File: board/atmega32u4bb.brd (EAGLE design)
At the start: 30.4 x 12.2 mm, 18 parts, among them X3 16MHz

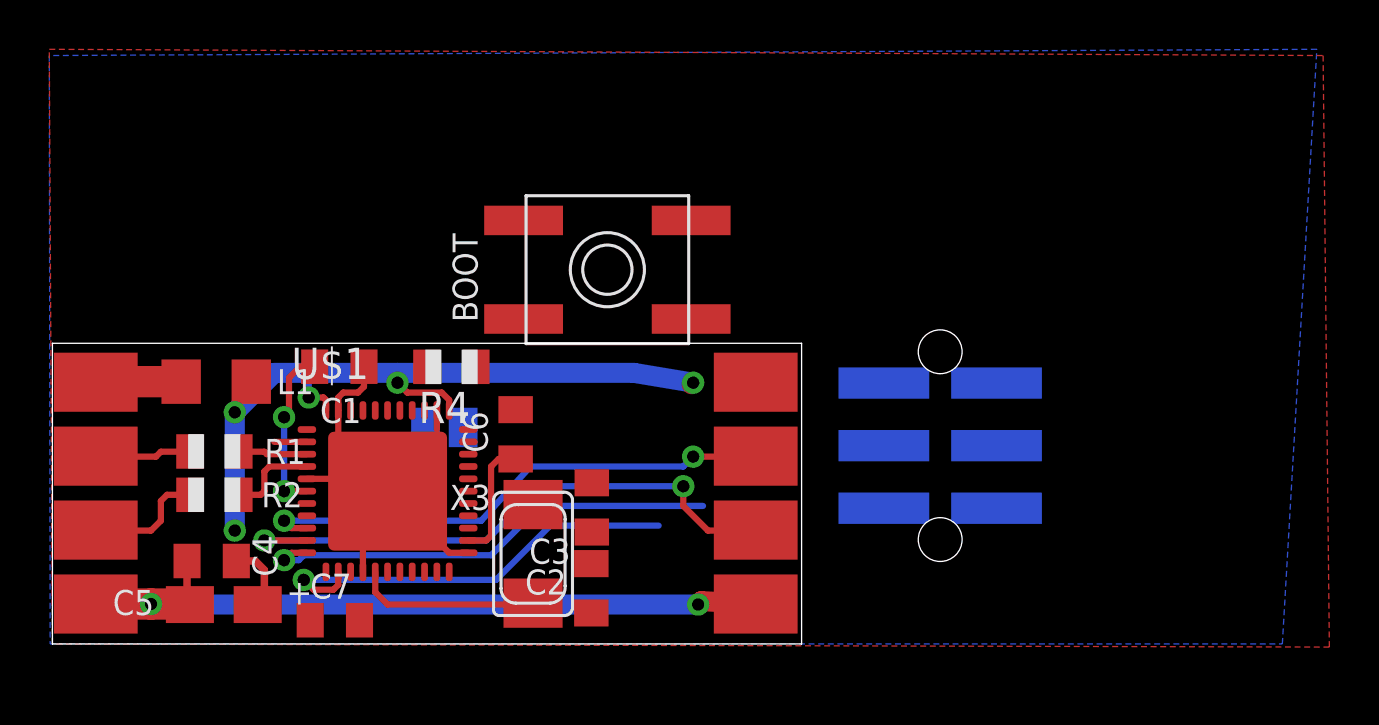
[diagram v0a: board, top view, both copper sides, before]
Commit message: V1 board design
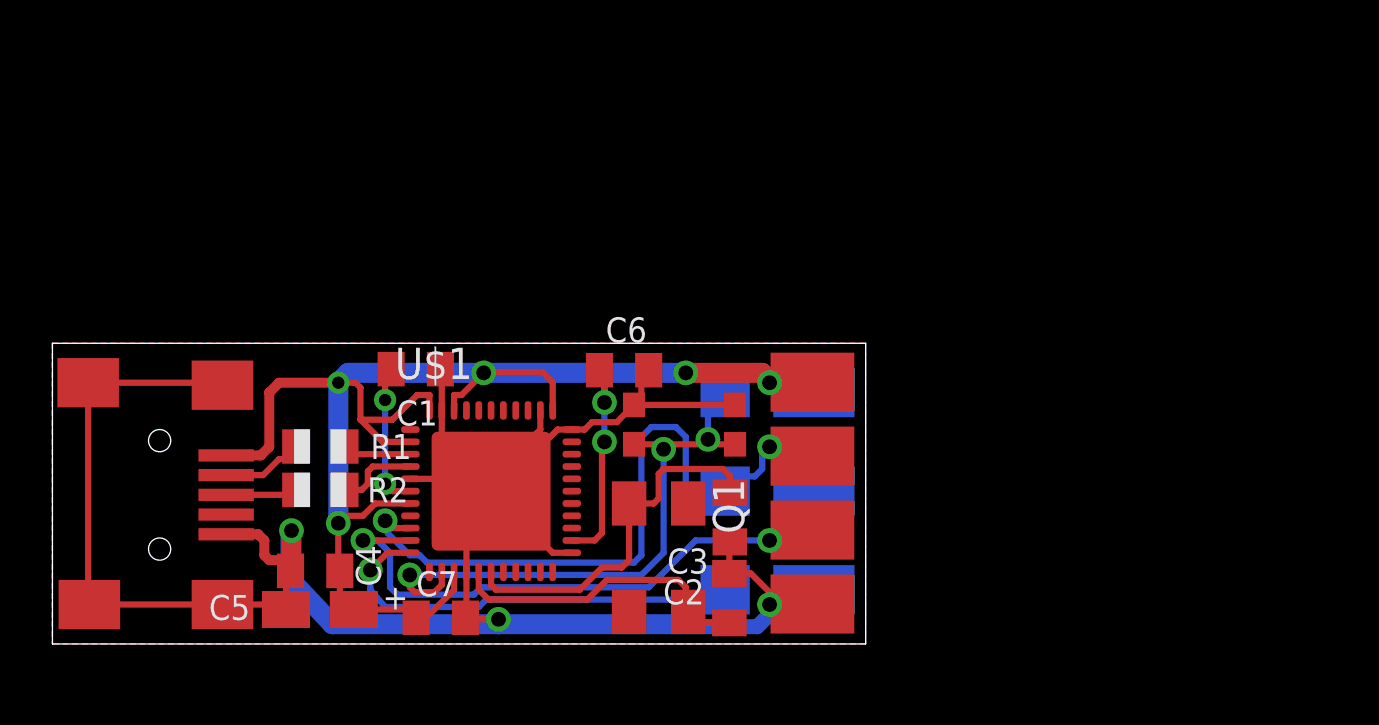
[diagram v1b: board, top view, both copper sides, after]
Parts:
- removed BOOT: EVQQ2, adaprog:EVQ-Q2
- removed ISP6: PINHD-2X3, adaprog:2X3SMT
- removed L1: 500mA, adafruit:R1206
- removed R4: 10K, adafruit:R0805
- removed SJ1: HWB, jumper:SJ
- removed U$5: USB_PADS, glowboard:PAD_CONNECTION
- removed X3: 16MHz, adaprog:NX5032
- added Q1: 16 MHz, glowboard:ABMM2_CRYSTAL
- added S1: Normally open, glowboard:KMR211G_SWITCH
- added U$2: MINI_USB, glowboard:MINI_USB_PADS
- added U$4: ICSP, glowboard:ICSP_PADS
- moved C2 5.61 mm to (27.5, 1.86)
- moved C3 5.61 mm to (27.5, 5.14)
- moved C6 5.11 mm to (23.2, 11.1), turned to 0 degrees
- moved R1 4.30 mm to (10.9, 8.01)
- moved R2 4.30 mm to (10.9, 6.25)
- moved C7 4.30 mm to (15.8, 1.06)
- moved C4 4.22 mm to (10.7, 2.97)
- moved U$1 4.20 mm to (17.8, 6.20)
- moved C5 3.91 mm to (10.9, 1.40)
- moved C1 3.10 mm to (14.7, 11.2)
- moved U$3 2.30 mm to (30.8, 6.02)
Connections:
- removed net AREF: U$1.42
- removed net HWB: R4.1, SJ1.1, U$1.33
- removed net N$1: L1.1, U$5.1
- net GND: now also S1.P$1, S1.P$2, U$1.33, U$2.P$5, U$2.P$6, U$2.P$7, U$2.P$8, U$2.P$9, U$4.GND; no longer BOOT.B, BOOT.B', ISP6.6, SJ1.2, U$5.4
- net MISO: now also U$4.MISO; no longer ISP6.1
- net MOSI: now also U$4.MOSI; no longer ISP6.4
- net N$2: now also U$2.P$3; no longer U$5.3
- net N$5: now also U$2.P$2; no longer U$5.2
- net N$8: now also Q1.P$3; no longer X3.P$2
- net N$9: now also Q1.P$1; no longer X3.P$1
- net RST: now also S1.P$3, S1.P$4, U$4.RST; no longer BOOT.A, BOOT.A', ISP6.5
- net SCK: now also U$4.SCK`; no longer ISP6.3
- net VCC: now also U$1.42, U$2.P$1, U$4.VCC; no longer ISP6.2, L1.2, R4.2
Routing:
- net GND: track 50.1 -> 96.0 mm, vias 2 -> 3
- net VCC: track 38.5 -> 71.5 mm, vias 5 -> 7
- net N$9: track 0.00 -> 15.0 mm
- net RST: track 17.5 -> 24.1 mm, vias 1 -> 3
- net SCK: track 21.3 -> 27.9 mm
- net N$8: track 7.18 -> 12.6 mm
- net N$1: track 3.47 -> 0.00 mm
- net MOSI: track 23.7 -> 26.4 mm
- net N$2: track 4.89 -> 2.87 mm
- net N$5: track 4.36 -> 3.30 mm
- net MISO: track 19.0 -> 18.0 mm
- net +3V3: track 6.84 -> 6.00 mm
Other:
- board size 30.4 x 12.2 mm -> 33 x 12.2 mm

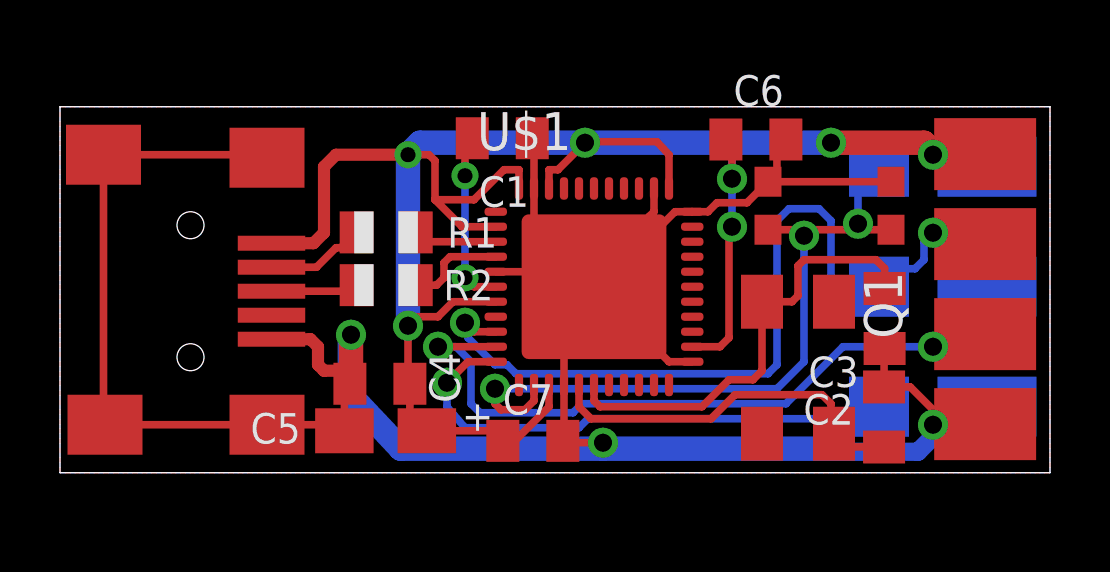
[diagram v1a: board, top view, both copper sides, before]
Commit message: Fix some errors
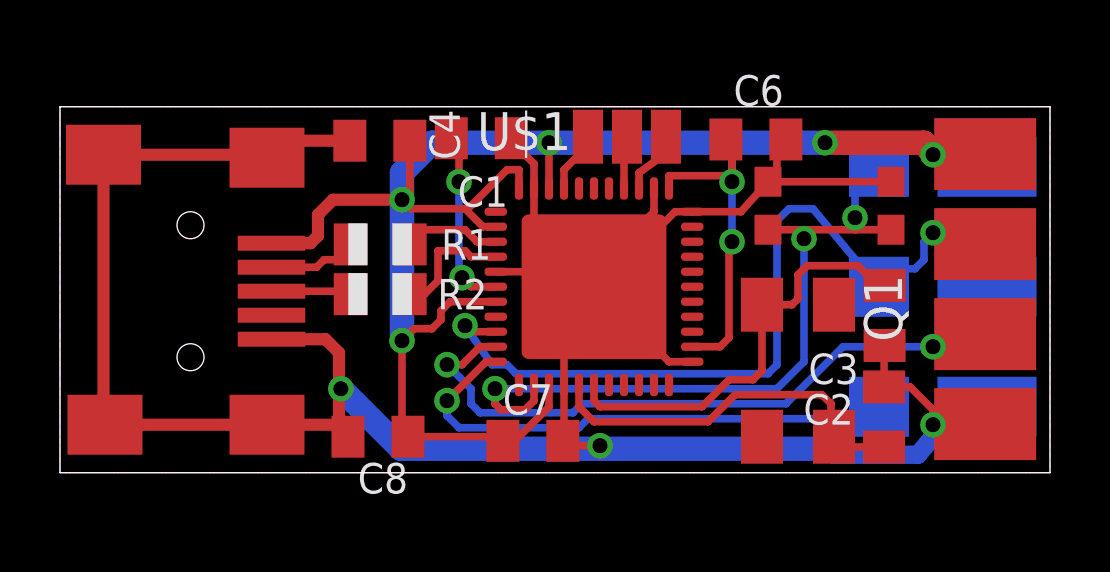
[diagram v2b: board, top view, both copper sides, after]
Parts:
- removed C5: 10uF, adafruit:A/3216-18R
- added C8: 0.1uF, adafruit:C0805K
- added U$5: EXPANSION_HEADER, glowboard:EXPANSION_HEADER
- moved C4 8.10 mm to (10.7, 11.1)
- moved C1 0.70 mm to (14.0, 11.2)
- moved R1 0.45 mm to (10.7, 7.61)
- moved R2 0.36 mm to (10.7, 5.95)
- moved Q1 0.10 mm to (24.6, 3.50)
- moved C3 0.10 mm to (27.5, 5.24)
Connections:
- new net N$1: U$1.41, U$5.P$1
- new net N$6: U$1.37, U$5.P$2
- new net N$7: U$1.36, U$5.P$3
- net GND: now also C8.2; no longer C5.-
- net VCC: now also C8.1; no longer C5.+
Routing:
- net N$7: track 0.00 -> 2.17 mm
- net N$1: track 0.00 -> 2.06 mm
- net VCC: track 71.5 -> 69.6 mm
- net N$6: track 0.00 -> 1.77 mm
- net MOSI: track 26.4 -> 25.2 mm
- net SCK: track 27.9 -> 26.8 mm
- net N$3: track 2.76 -> 3.59 mm
- net N$9: track 15.0 -> 14.2 mm
- net N$4: track 3.34 -> 4.12 mm
